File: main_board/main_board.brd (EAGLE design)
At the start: 32.5 x 32.5 mm, 15 parts, among them Q1 FC-12M, U1 MDBT40SMD, U2 MPU-9250

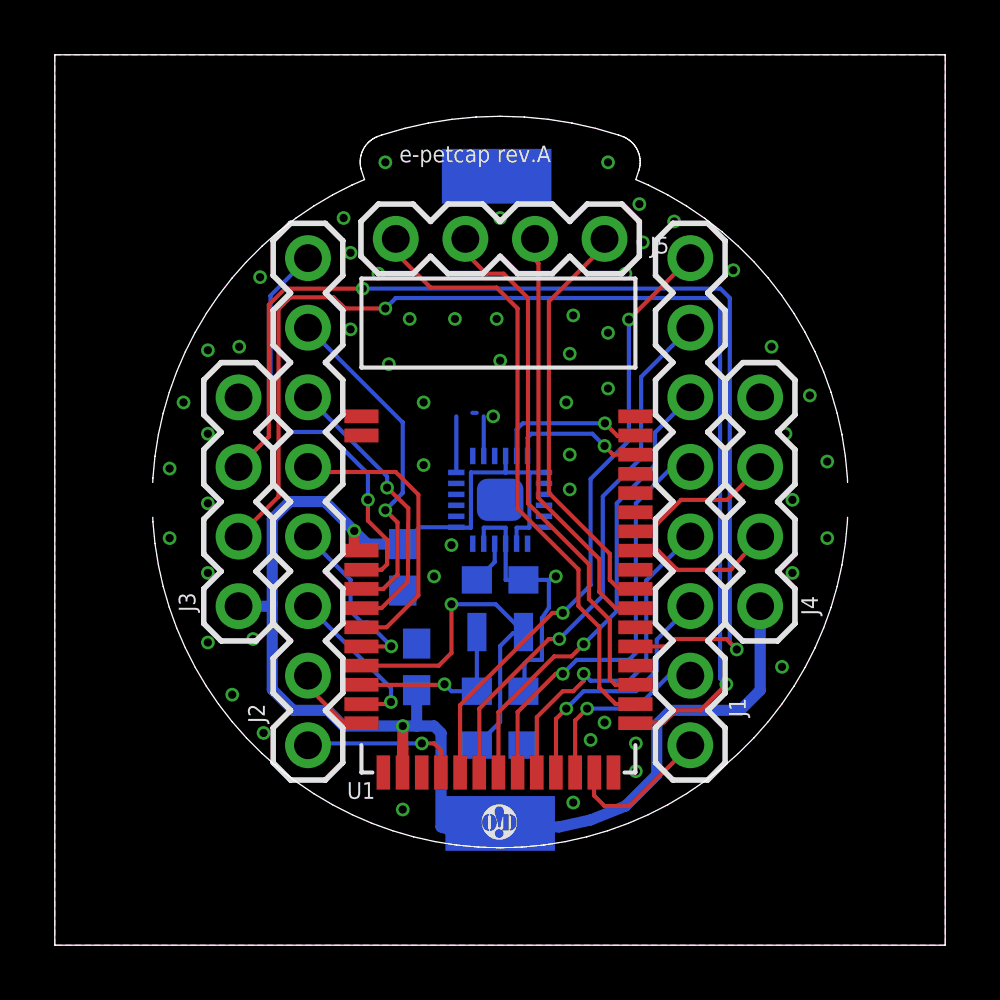
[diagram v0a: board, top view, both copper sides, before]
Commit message: MDBT42
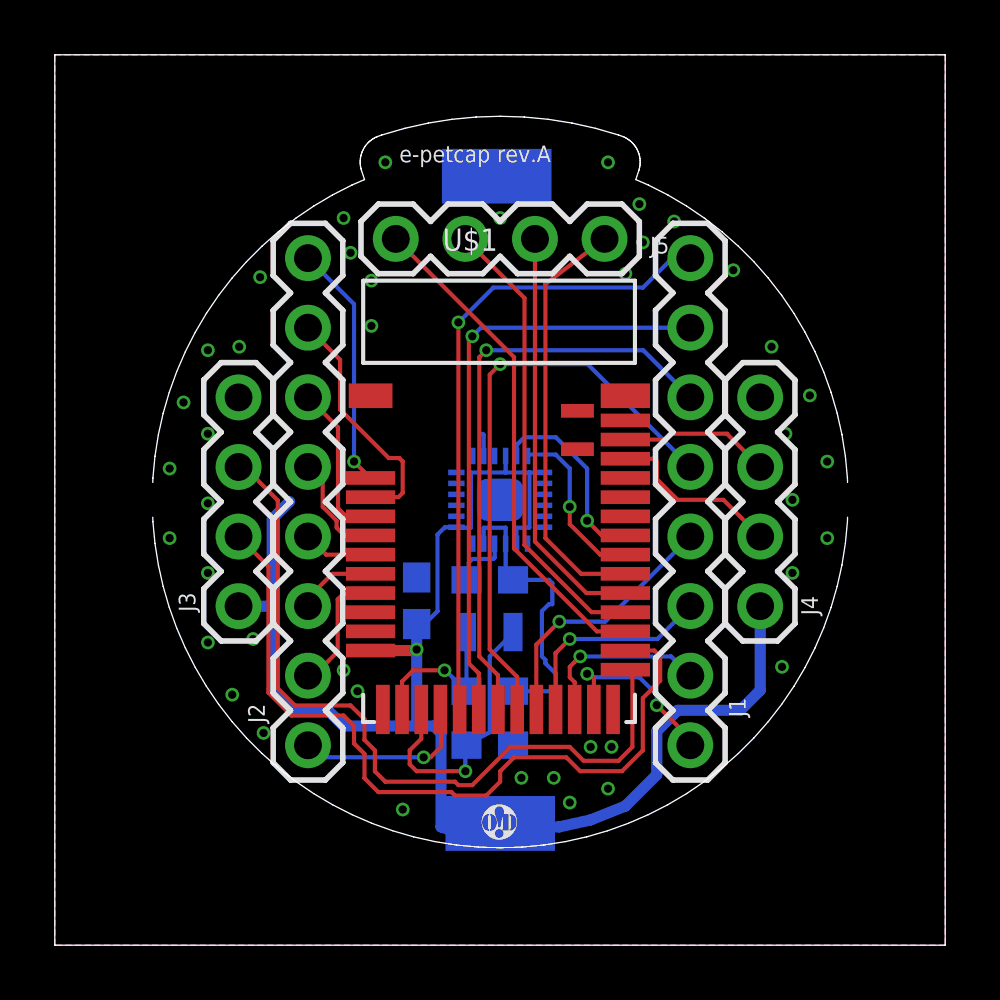
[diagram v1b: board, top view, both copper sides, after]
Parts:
- removed C5: .1uF, SparkFun-Capacitors:0603-CAP
- removed U1: MDBT40SMD, MDBT40:MDBT40
- added U$1: MDBT42SMD, MDBT42:MDBT42
- C3: value 1uF -> 10uF
- moved C3 2.41 mm to (13.2, 12.6)
- moved C1 0.38 mm to (15.9, 13.3)
- moved C6 0.38 mm to (15.9, 9.27)
- moved C7 0.38 mm to (15.9, 7.30)
- moved Q1 0.38 mm to (15.9, 11.4)
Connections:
- removed net LED4: U1.37
- new net LED0: U$1.34
- new net LED1: U$1.33
- new net NRESET: U$1.35
- net A0: now also U$1.16; no longer U1.17
- net A1: now also U$1.17; no longer U1.18
- net A2: now also U$1.18; no longer U1.19
- net A3: now also U$1.19; no longer U1.20
- net A4: now also U$1.20; no longer U1.21
- net A5: now also U$1.21; no longer U1.22
- net A6: now also U$1.22; no longer U1.23
- net A7: now also U$1.23; no longer U1.24
- net D0: now also U$1.2; no longer U1.4
- net D1: now also U$1.3; no longer U1.5
- net D2: now also U$1.4; no longer U1.6
- net D3: now also U$1.5; no longer U1.7
- net D4: now also U$1.6; no longer U1.8
- net D5: now also U$1.7; no longer U1.11
- net D6: now also U$1.8; no longer U1.12
- net D7: now also U$1.15; no longer U1.16
- net GND: now also U$1.1, U$1.12, U$1.24, U$1.39; no longer C5.2, U1.1, U1.13, U1.2, U1.25, U1.42
- net N$2: now also U$1.14; no longer U1.9
- net N$3: now also U$1.13; no longer U1.10
- net RX: now also U$1.25; no longer U1.30
- net SPI_MISO: now also U$1.29; no longer U1.32
- net SPI_MOSI: now also U$1.27; no longer U1.27
- net SPI_SCK: now also U$1.28; no longer U1.28
- net SPI_SS: now also U$1.30; no longer U1.33
- net SWCLK: now also J4.2, U$1.36; no longer J4.3, U1.36
- net SWDIO: now also J4.3, U$1.37; no longer J4.2, U1.35
- net TWI_SCL: now also U$1.32; no longer U1.41
- net TWI_SDA: now also U$1.31; no longer U1.40
- net TX: now also U$1.26; no longer U1.26
- net VCC: now also U$1.11; no longer C5.1, U1.14, U1.3
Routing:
- net TX: track 43.5 -> 28.6 mm, vias 2 -> 0
- net RX: track 40.5 -> 28.0 mm, vias 2 -> 0
- net D3: track 10.7 -> 3.31 mm
- net D0: track 15.3 -> 8.97 mm
- net A3: track 15.4 -> 21.7 mm
- net A2: track 17.0 -> 21.7 mm
- net D2: track 10.4 -> 5.81 mm, vias 1 -> 0
- net SPI_MOSI: track 22.4 -> 18.4 mm
- net D4: track 6.48 -> 2.56 mm, vias 1 -> 0
- net D1: track 12.4 -> 8.92 mm, vias 1 -> 0
- net N$2: track 13.3 -> 10.3 mm
- net D5: track 5.91 -> 2.94 mm, vias 1 -> 0
- net SPI_SCK: track 19.6 -> 16.8 mm
- net A4: track 12.5 -> 9.62 mm
- net A1: track 19.6 -> 21.9 mm
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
